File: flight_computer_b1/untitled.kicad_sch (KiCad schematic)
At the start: 14 parts, among them Q3 NMOS, Q4 NMOS

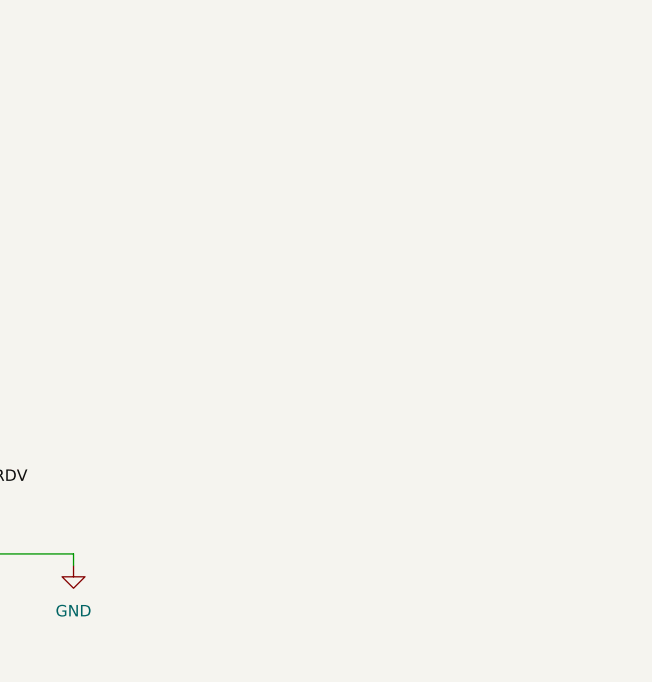
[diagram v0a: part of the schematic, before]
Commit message: Fixed Schematic
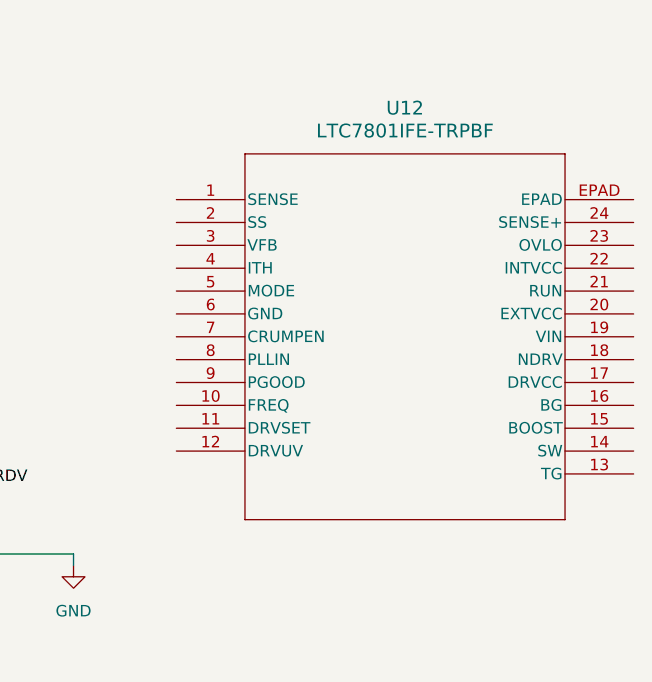
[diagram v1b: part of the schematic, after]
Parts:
- added U12: LTC7801IFE-TRPBF, FE_24_ADI, symbol LTC7801:LTC7801IFE-TRPBF
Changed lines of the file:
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@@
+	)
+	(symbol
+		(lib_id "LTC7801:LTC7801IFE-TRPBF")
+		(at 167.64 77.47 0)
+		(unit 1)
+		(exclude_from_sim no)
+		(in_bom yes)
+		(on_board yes)
+		(dnp no)
+		(fields_autoplaced yes)
+		(property "Reference" "U12"
+			(at 193.04 67.31 0)
+			(effects
+				(font
+					(size 1.524 1.524)
+				)
+			)
+		)
+		(property "Value" "LTC7801IFE-TRPBF"
+			(at 193.04 69.85 0)
+			(effects
+				(font
+					(size 1.524 1.524)
+				)
+			)
+		)
+		(property "Footprint" "FE_24_ADI"
+			(at 167.64 77.47 0)
+			(effects
+				(font
+					(size 1.27 1.27)
+					(italic yes)
+				)
+				(hide yes)
+			)
+		)
+		(property "Datasheet" "https://www.analog.com/media/en/technical-documentation/data-sheets/ltc7801.pdf"
+			(at 167.64 77.47 0)
+			(effects
+				(font
+					(size 1.27 1.27)
+					(italic yes)
+				)
+				(hide yes)
+			)
+		)
+		(property "Description" ""
+			(at 167.64 77.47 0)
+			(effects
+				(font
+					(size 1.27 1.27)
+				)
+				(hide yes)
+			)
+		)
+		(pin "1"
+		)
+		(pin "14"
+		)
+		(pin "13"
+		)
+		(pin "17"
+		)
+		(pin "16"
+		)
+		(pin "15"
+		)
+		(pin "20"
+		)
+		(pin "19"
+		)
+		(pin "18"
+		)
+		(pin "23"
+		)
+		(pin "22"
+		)
+		(pin "21"
+		)
+		(pin "10"
+		)
+		(pin "11"
+		)
+		(pin "12"
+		)
+		(pin "EPAD"
+		)
+		(pin "24"
+		)
+		(pin "3"
+		)
+		(pin "4"
+		)
+		(pin "5"
+		)
+		(pin "6"
+		)
+		(pin "7"
+		)
+		(pin "8"
+		)
+		(pin "9"
+		)
+		(pin "2"
+		)
+		(instances
+			(project ""
+				(path "/b71a7b79-cdb5-4e38-a72c-0daaa3474f05/dafce160-673b-4056-acfb-f0ec341d8d32"
+					(reference "U12")
+					(unit 1)
+				)
+			)
+		)
 	)
 	(symbol
